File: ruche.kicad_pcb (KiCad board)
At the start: 2 copper layers, 92.8 x 99.9 mm, 195 parts, among them IC1 CN3791, IC2 MAX17048G+, IC3 L86-M33, IC4 SHT41-AD1B-R3, IC5 HX711, IC6 HX711, IC7 HX711, IC8 HX711, IC9 FS312F-G, J1 Conn_01x02, J10 Conn_01x04, J11 Conn_01x04, J12 Conn_01x04, J13 Micro_SD_Card, J14 Conn_01x03, J15 Conn_01x04, J16 Conn_01x04, J17 Conn_01x04, J18 Conn_01x04, J19 Conn_01x02, J2 Conn_01x04, J20 USB_C_Receptacle_USB2.0 USB41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, J21 Conn_01x02, J3 Conn_01x03, J4 Conn_01x02, J5 Conn_01x04, J6 Conn_01x02, J7 Conn_01x02, J8 Conn_01x03, J9 Conn_01x03, Q1 AO3401A, Q2 MMBT4403, Q3 MMBT4403, Q4 MMBT4403, Q5 MMBT4403, Q6 UMH3N, Q7 DMG2301L, Q8 FS8205, SW1 SW_Push, SW2 SW_Push, U1 CP2102N-A02-GQFN24, U2 MS5611-01BA, U3 XC6220B331MR, U4 TCA9548APWR, U5 XC6220B331MR, U6 Heltec_Wireless_shell_V3, U7 1043, U9 XC6220B331MR

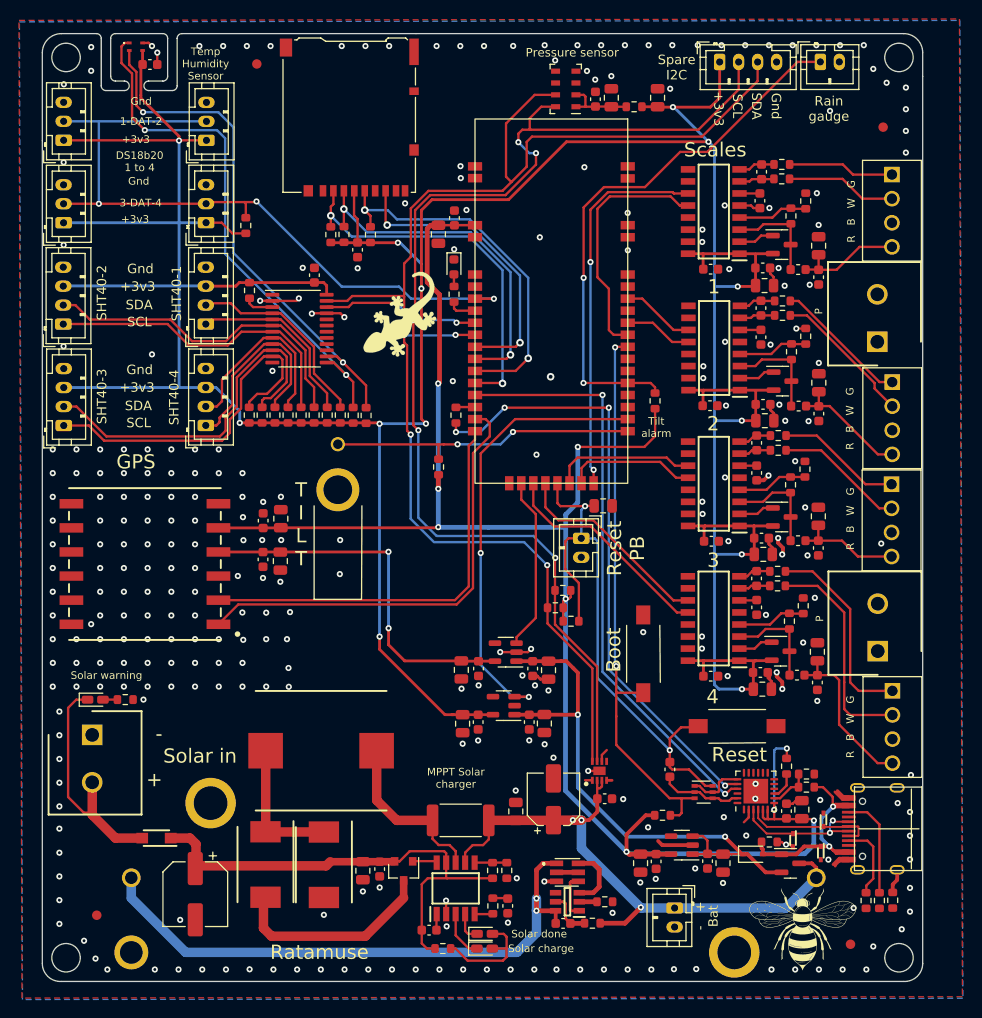
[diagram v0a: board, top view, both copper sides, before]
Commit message: update
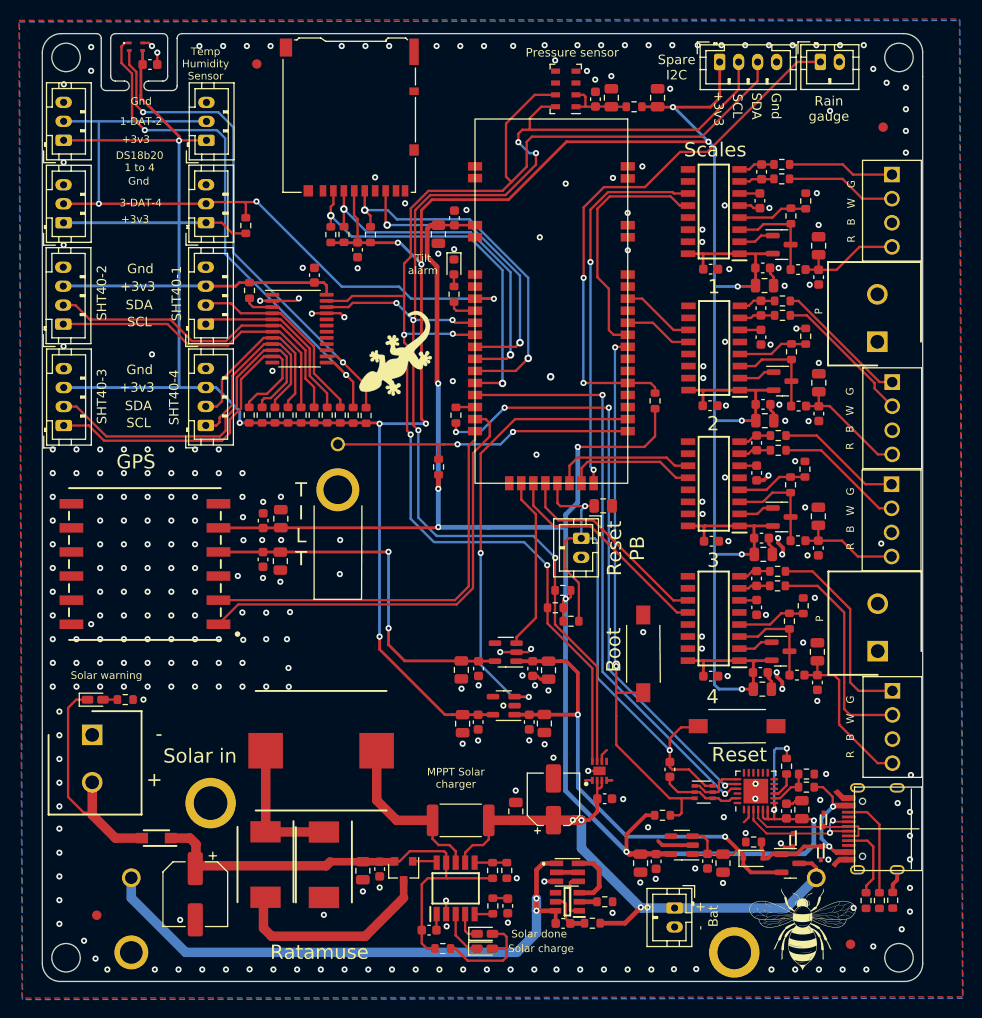
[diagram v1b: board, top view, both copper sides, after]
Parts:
- moved G*** 4.15 mm to (123.7, 103.2)
- moved R49 1.66 mm to (161.5, 154.3), turned to 180 degrees
- moved D14 0.44 mm to (161.4, 156.0)
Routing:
- net VCC: track 401.7 -> 399.2 mm
- net VBUS: track 25.3 -> 25.9 mm
- net VBAT: track 62.9 -> 63.5 mm, vias 3 -> 4
- net GND: track 54.4 -> 54.2 mm, vias 297 -> 301

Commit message: Revert "update"
This reverts commit 9afc669c055c7e8087787cb6fdf10dddd7845243.
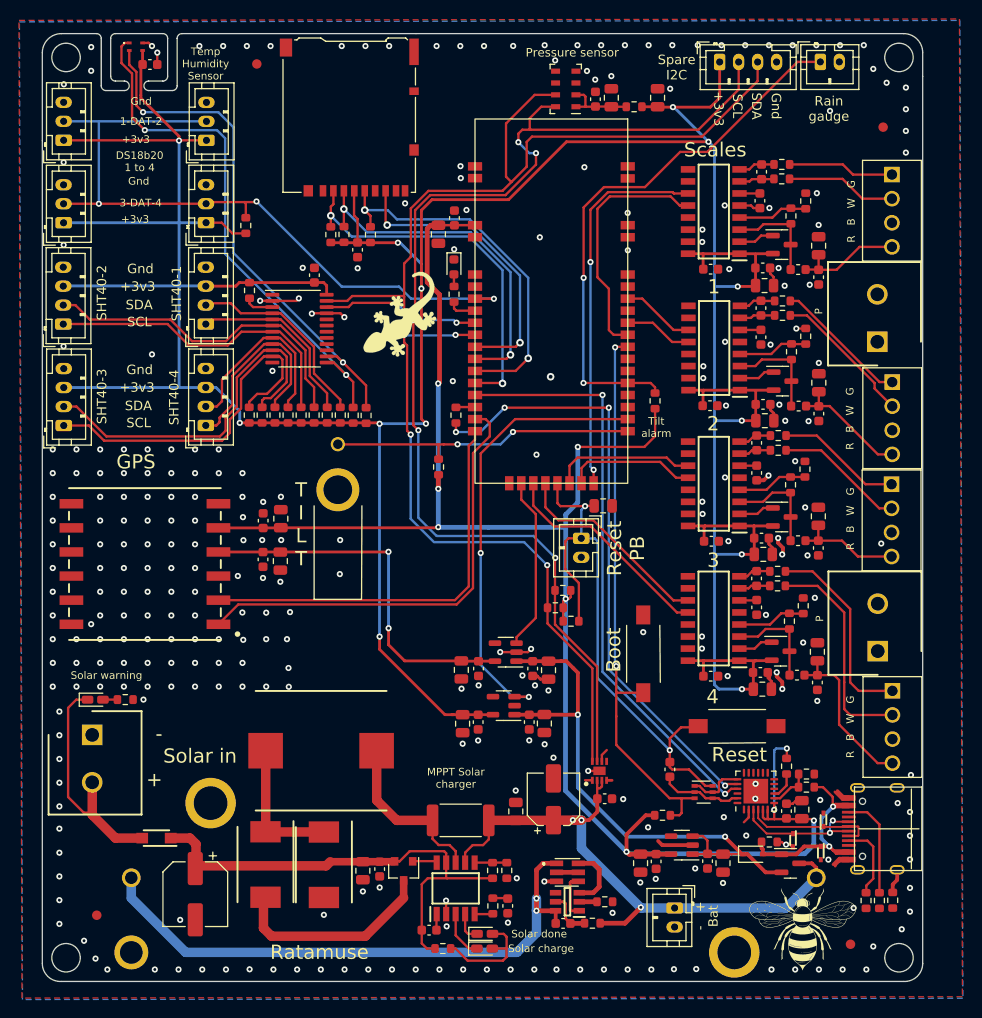
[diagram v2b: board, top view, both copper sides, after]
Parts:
- moved G*** 4.15 mm to (124.1, 99.0)
- moved R49 1.66 mm to (163.1, 154.3), turned to 0 degrees
- moved D14 0.44 mm to (161.4, 155.6)
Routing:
- net VCC: track 399.2 -> 401.7 mm
- net VBUS: track 25.9 -> 25.3 mm
- net VBAT: track 63.5 -> 62.9 mm, vias 4 -> 3
- net GND: track 54.2 -> 54.4 mm, vias 301 -> 297
